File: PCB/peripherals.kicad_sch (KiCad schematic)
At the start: 19 parts, among them J1 Conn_01x03_Pin, J2 Conn_01x02_Pin, J3 Conn_01x02_Pin, J4 Conn_01x03_Pin, J5 Conn_01x03_Pin, J6 Conn_01x03_Pin, J7 Conn_01x07_Pin, J8 Conn_01x08_Socket, U2 MPU-6050

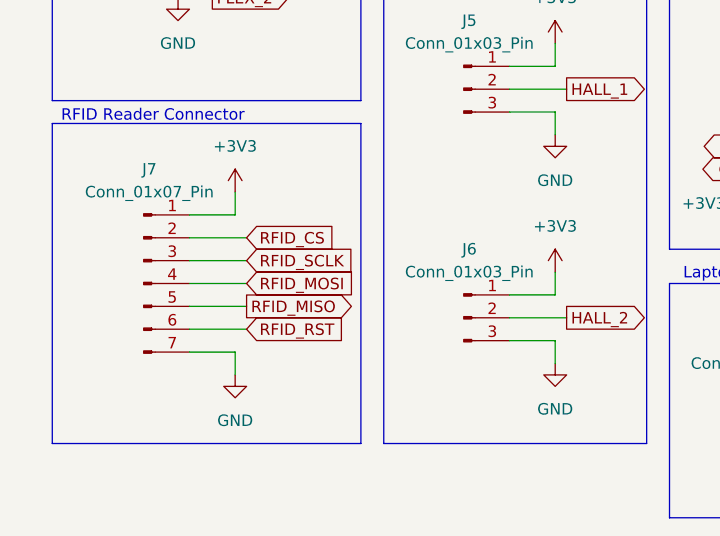
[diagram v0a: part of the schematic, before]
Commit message: place and route connectors, add edges
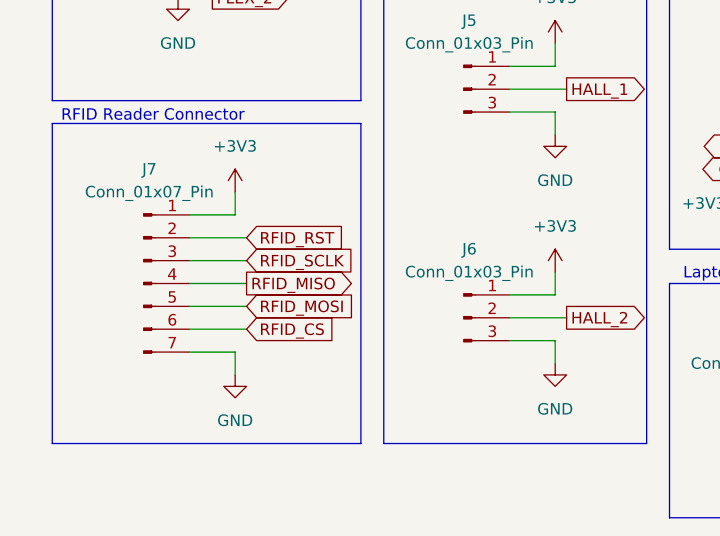
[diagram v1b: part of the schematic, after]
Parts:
- J1, J4, J5, J6: footprint Connector_JST:JST_VH_B3P-VH_1x03_P3.96mm_Vertical -> Connector_JST:JST_VH_B3PS-VH_1x03_P3.96mm_Horizontal
- J2, J3: footprint Connector_JST:JST_VH_B2P-VH_1x02_P3.96mm_Vertical -> Connector_JST:JST_VH_B2PS-VH_1x02_P3.96mm_Horizontal
- J7: footprint Connector_JST:JST_VH_B7P-VH_1x07_P3.96mm_Vertical -> Connector_JST:JST_VH_B7PS-VH_1x07_P3.96mm_Horizontal
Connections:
- net RFID_CS: now also J7.6 (Pin_6); no longer J7.2 (Pin_2)
- net RFID_MISO: now also J7.4 (Pin_4); no longer J7.5 (Pin_5)
- net RFID_MOSI: now also J7.5 (Pin_5); no longer J7.4 (Pin_4)
- net RFID_RST: now also J7.2 (Pin_2); no longer J7.6 (Pin_6)
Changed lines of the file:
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@@
 	(global_label "RFID_RST"
 		(shape input)
-		(at 39.37 165.1 0)
+		(at 39.37 154.94 0)
 		(fields_autoplaced yes)
 		(effects
@@
 		)
 		(property "Intersheetrefs" "${INTERSHEET_REFS}"
-			(at 51.0033 165.1 0)
+			(at 50.0357 154.94 0)
 			(effects
 				(font
@@
 	(global_label "RFID_MISO"
 		(shape output)
-		(at 39.37 162.56 0)
+		(at 39.37 160.02 0)
 		(fields_autoplaced yes)
 		(effects
@@
 		)
 		(property "Intersheetrefs" "${INTERSHEET_REFS}"
-			(at 52.1524 162.56 0)
+			(at 52.1524 160.02 0)
 			(effects
 				(font
@@
 	(global_label "RFID_MOSI"
 		(shape input)
-		(at 39.37 160.02 0)
+		(at 39.37 162.56 0)
 		(fields_autoplaced yes)
 		(effects
@@
 		)
 		(property "Intersheetrefs" "${INTERSHEET_REFS}"
-			(at 52.1524 160.02 0)
+			(at 52.1524 162.56 0)
 			(effects
 				(font
@@
 	(global_label "RFID_CS"
 		(shape input)
-		(at 39.37 154.94 0)
+		(at 39.37 165.1 0)
 		(fields_autoplaced yes)
 		(effects
@@
 		)
 		(property "Intersheetrefs" "${INTERSHEET_REFS}"
-			(at 50.0357 154.94 0)
+			(at 51.0033 165.1 0)
 			(effects
 				(font
@@
 			)
 		)
-		(property "Footprint" "Connector_JST:JST_VH_B3P-VH_1x03_P3.96mm_Vertical"
+		(property "Footprint" "Connector_JST:JST_VH_B3PS-VH_1x03_P3.96mm_Horizontal"
 			(at 95.25 173.99 0)
 			(effects
@@
 			)
 		)
-		(property "Footprint" "Connector_JST:JST_VH_B2P-VH_1x02_P3.96mm_Vertical"
+		(property "Footprint" "Connector_JST:JST_VH_B2PS-VH_1x02_P3.96mm_Horizontal"
 			(at 25.4 104.14 0)
 			(effects
@@
 			)
 		)
-		(property "Footprint" "Connector_JST:JST_VH_B2P-VH_1x02_P3.96mm_Vertical"
+		(property "Footprint" "Connector_JST:JST_VH_B2PS-VH_1x02_P3.96mm_Horizontal"
 			(at 25.4 123.19 0)
 			(effects
@@
 			)
 		)
-		(property "Footprint" "Connector_JST:JST_VH_B7P-VH_1x07_P3.96mm_Vertical"
+		(property "Footprint" "Connector_JST:JST_VH_B7PS-VH_1x07_P3.96mm_Horizontal"
 			(at 27.94 160.02 0)
 			(effects
@@
 			)
 		)
-		(property "Footprint" "Connector_JST:JST_VH_B3P-VH_1x03_P3.96mm_Vertical"
+		(property "Footprint" "Connector_JST:JST_VH_B3PS-VH_1x03_P3.96mm_Horizontal"
 			(at 63.5 138.43 0)
 			(effects
@@
 			)
 		)
-		(property "Footprint" "Connector_JST:JST_VH_B3P-VH_1x03_P3.96mm_Vertical"
+		(property "Footprint" "Connector_JST:JST_VH_B3PS-VH_1x03_P3.96mm_Horizontal"
 			(at 63.5 163.83 0)
 			(effects
@@
 			)
 		)
-		(property "Footprint" "Connector_JST:JST_VH_B3P-VH_1x03_P3.96mm_Vertical"
+		(property "Footprint" "Connector_JST:JST_VH_B3PS-VH_1x03_P3.96mm_Horizontal"
 			(at 62.23 107.95 0)
 			(effects
